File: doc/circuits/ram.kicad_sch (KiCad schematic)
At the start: 12 parts, among them U1 AS6C4008-55PCN, U10 74LS04, U11 74LS08, U12 74LS04, U2 AS6C4008-55PCN, U3 74HC245, U4 74HC245, U5 74LS04, U6 74HC86, U7 74HC86, U8 74LS08, U9 74LS08

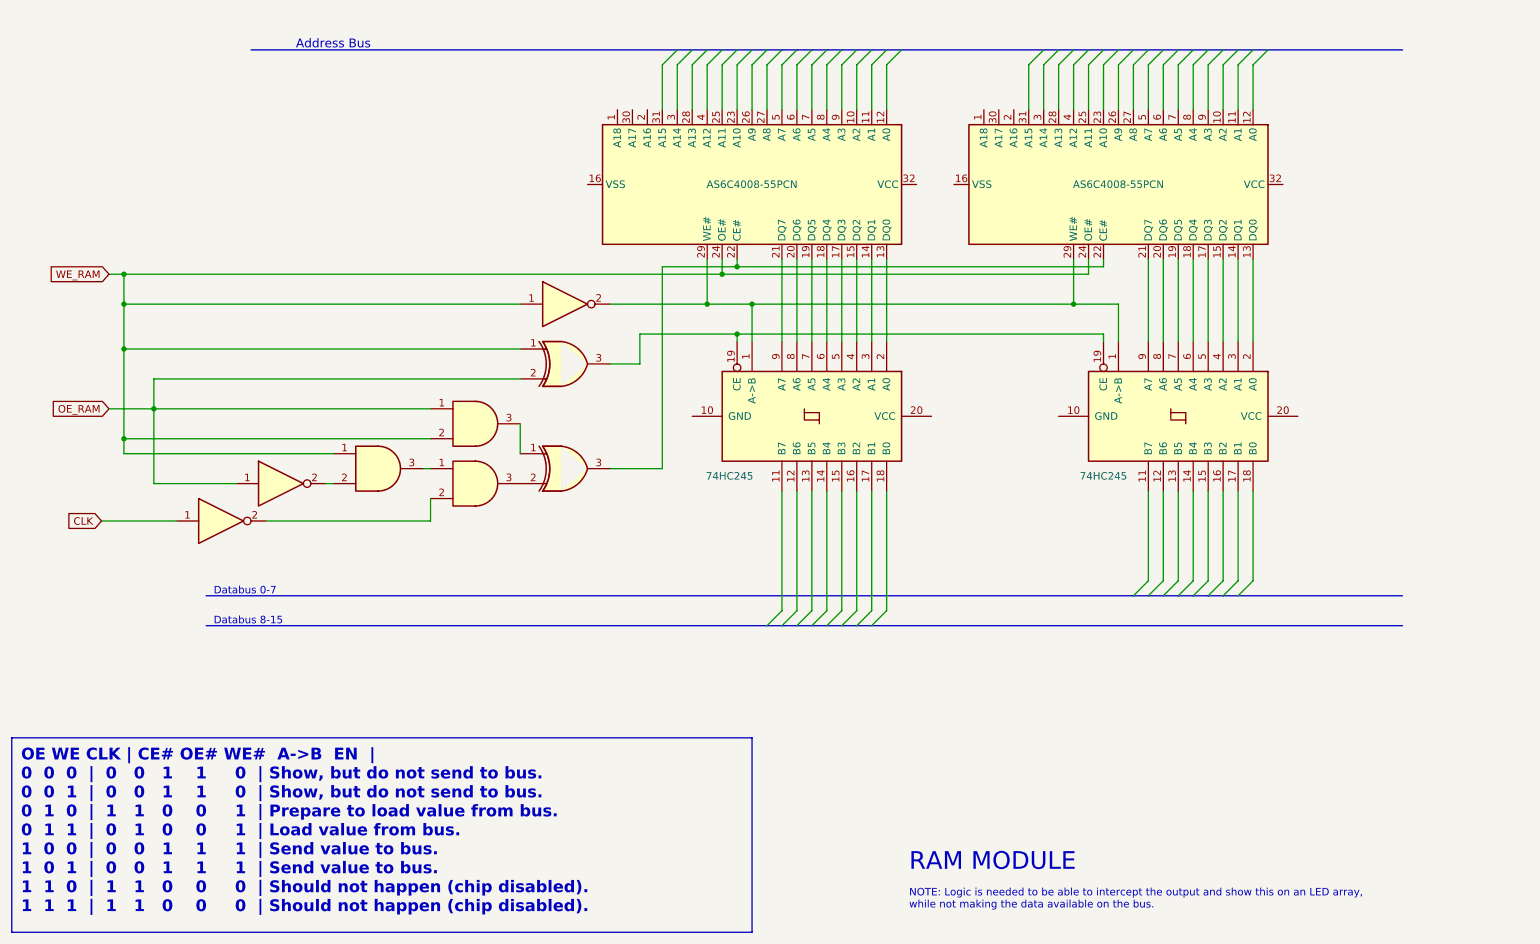
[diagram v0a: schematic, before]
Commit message: Updated schematics
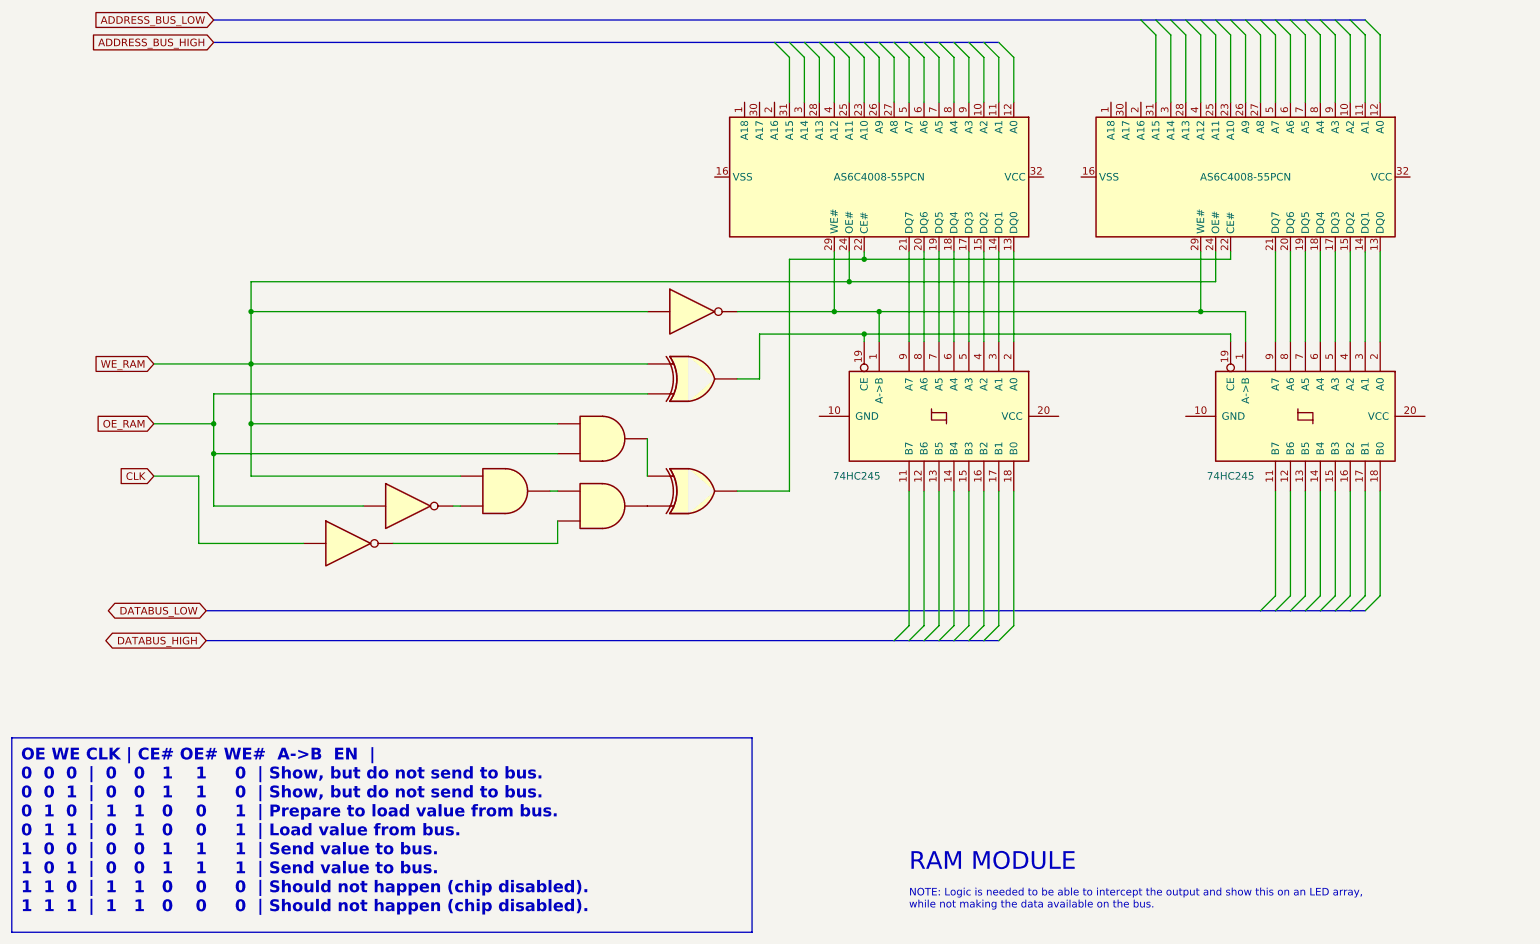
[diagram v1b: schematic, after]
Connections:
- net OE_RAM: now also U8.2; no longer U8.1
- net WE_RAM: now also U8.1; no longer U8.2
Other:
- note removed: "Address Bus"
- note removed: "Databus 0-7"
- note removed: "Databus 8-15"
